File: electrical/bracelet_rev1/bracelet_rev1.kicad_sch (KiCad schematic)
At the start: 0 parts

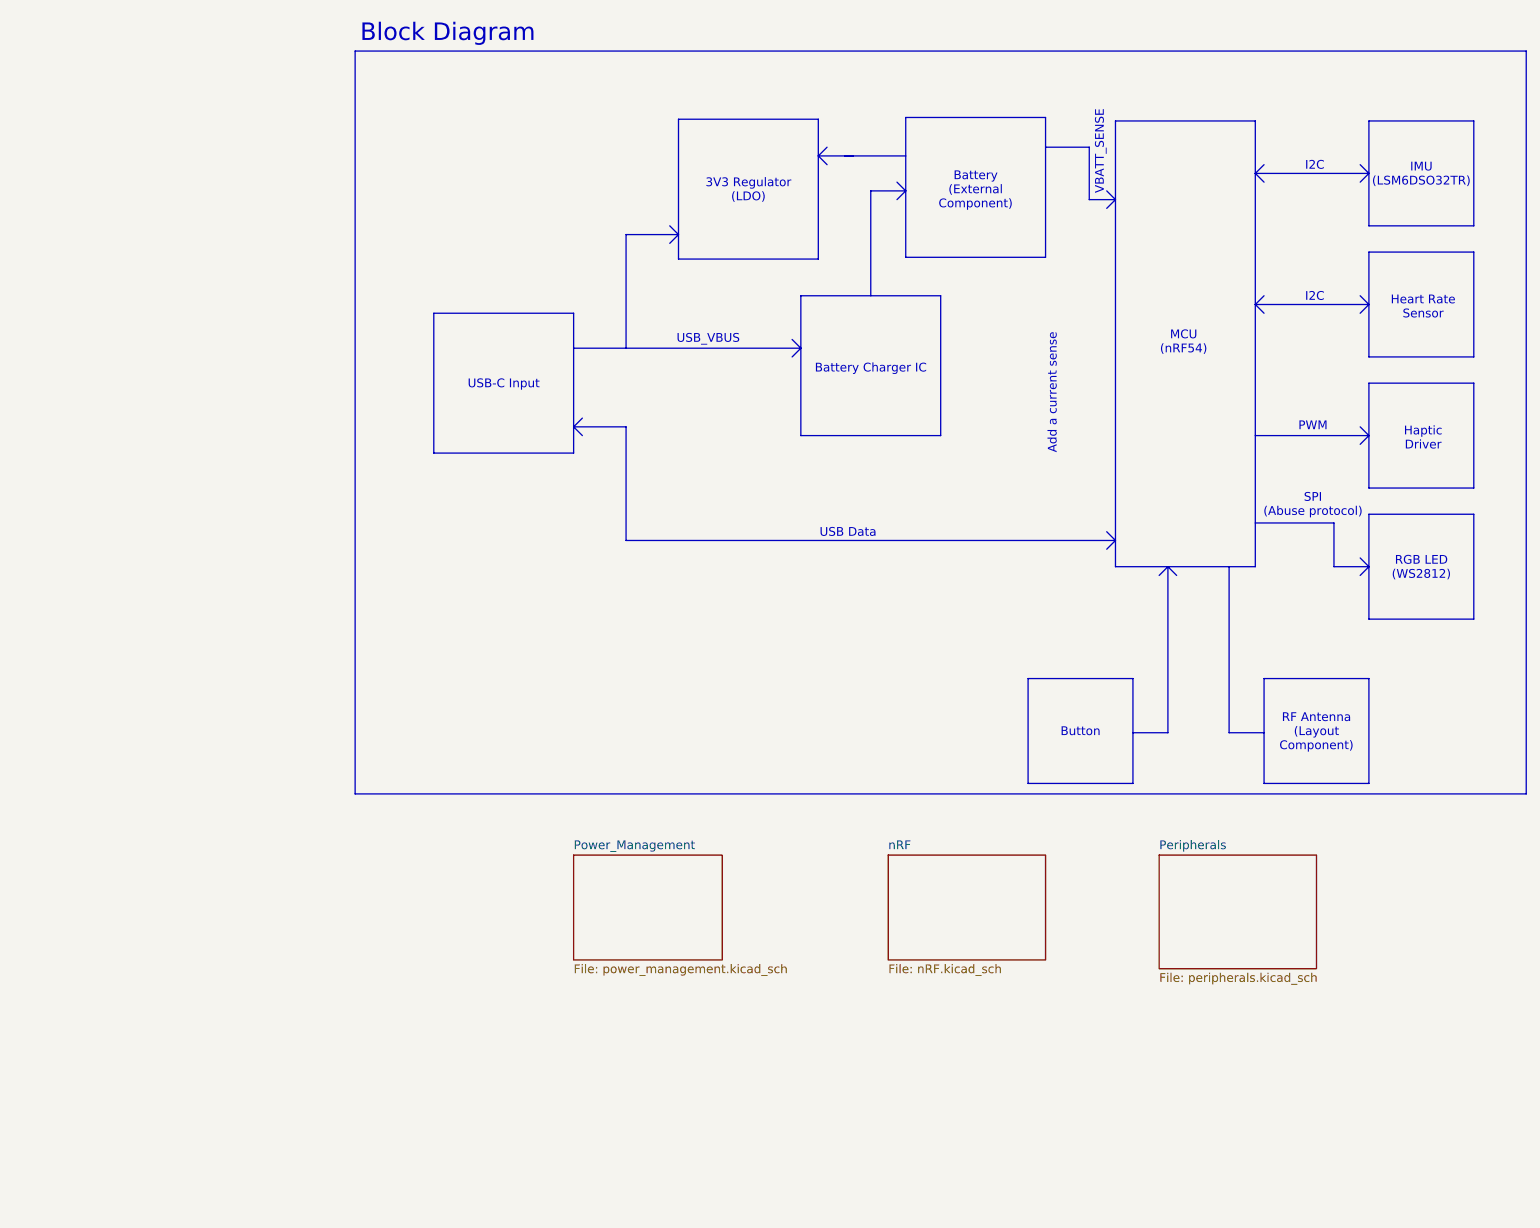
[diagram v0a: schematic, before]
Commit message: Mostly finihsed hopefully but still needs clean up anyway
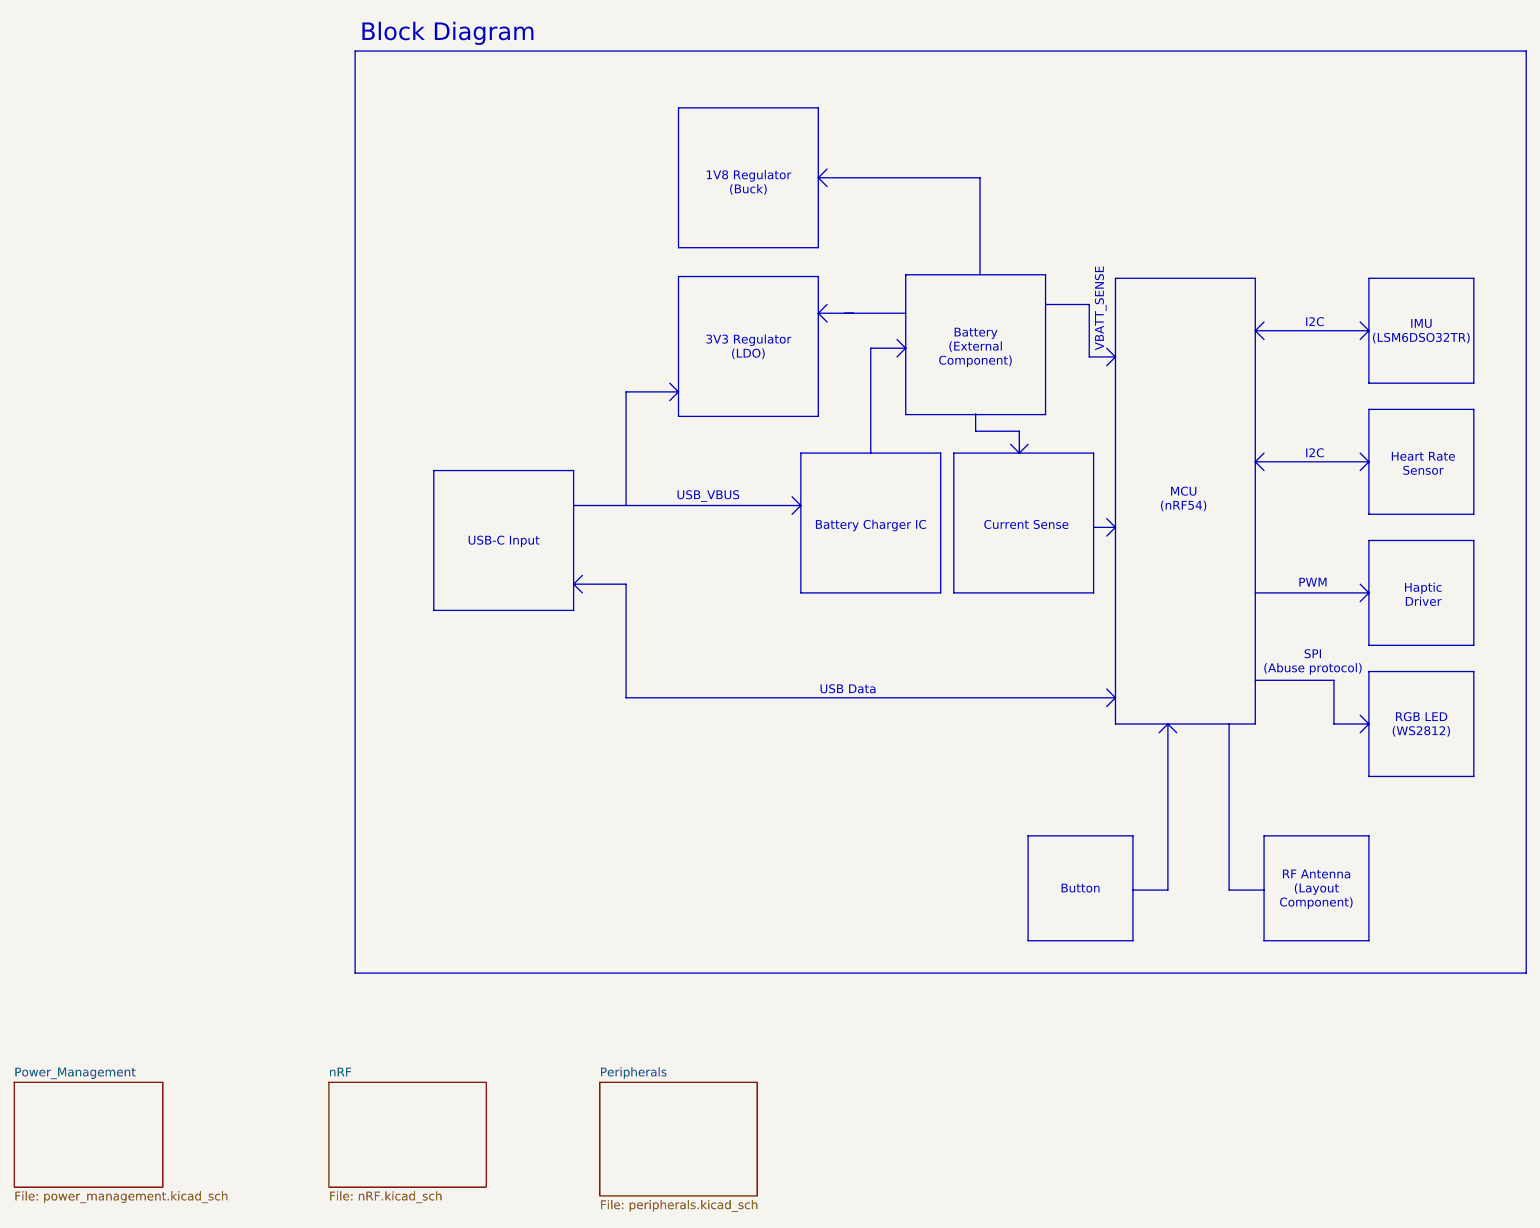
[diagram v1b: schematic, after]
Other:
- note added: "1V8 Regulator (Buck)"
- note added: "Current Sense"
- note removed: "Add a current sense"
